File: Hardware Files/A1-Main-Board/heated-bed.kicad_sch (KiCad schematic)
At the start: 16 parts, among them J11 FPC2, J8 FPC_CON, J9 FPC1, Q1 NMOS

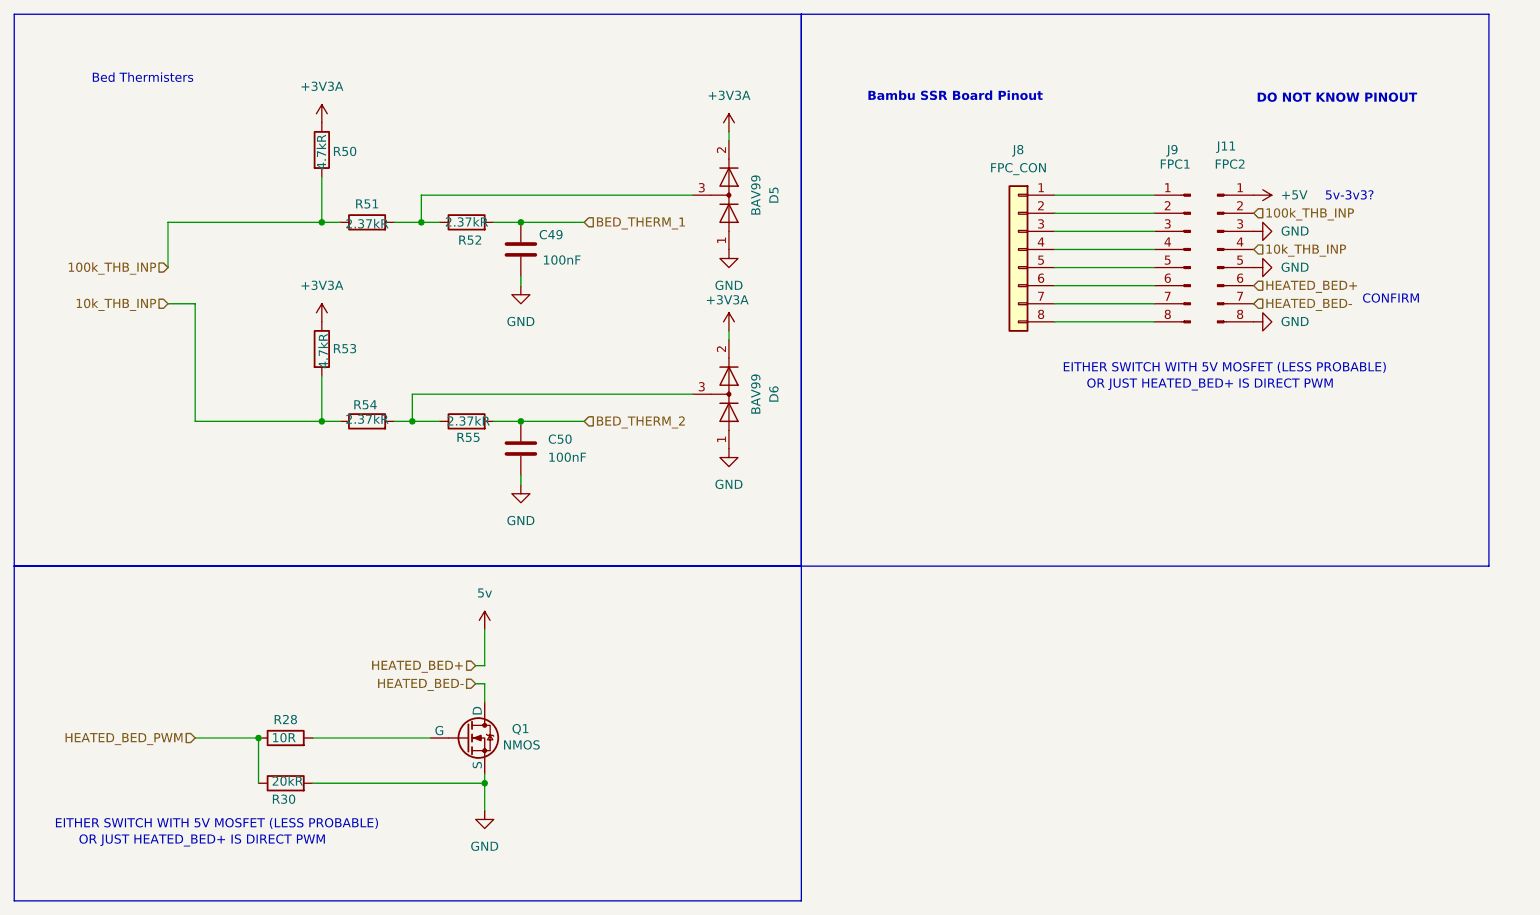
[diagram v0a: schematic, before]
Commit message: e
e
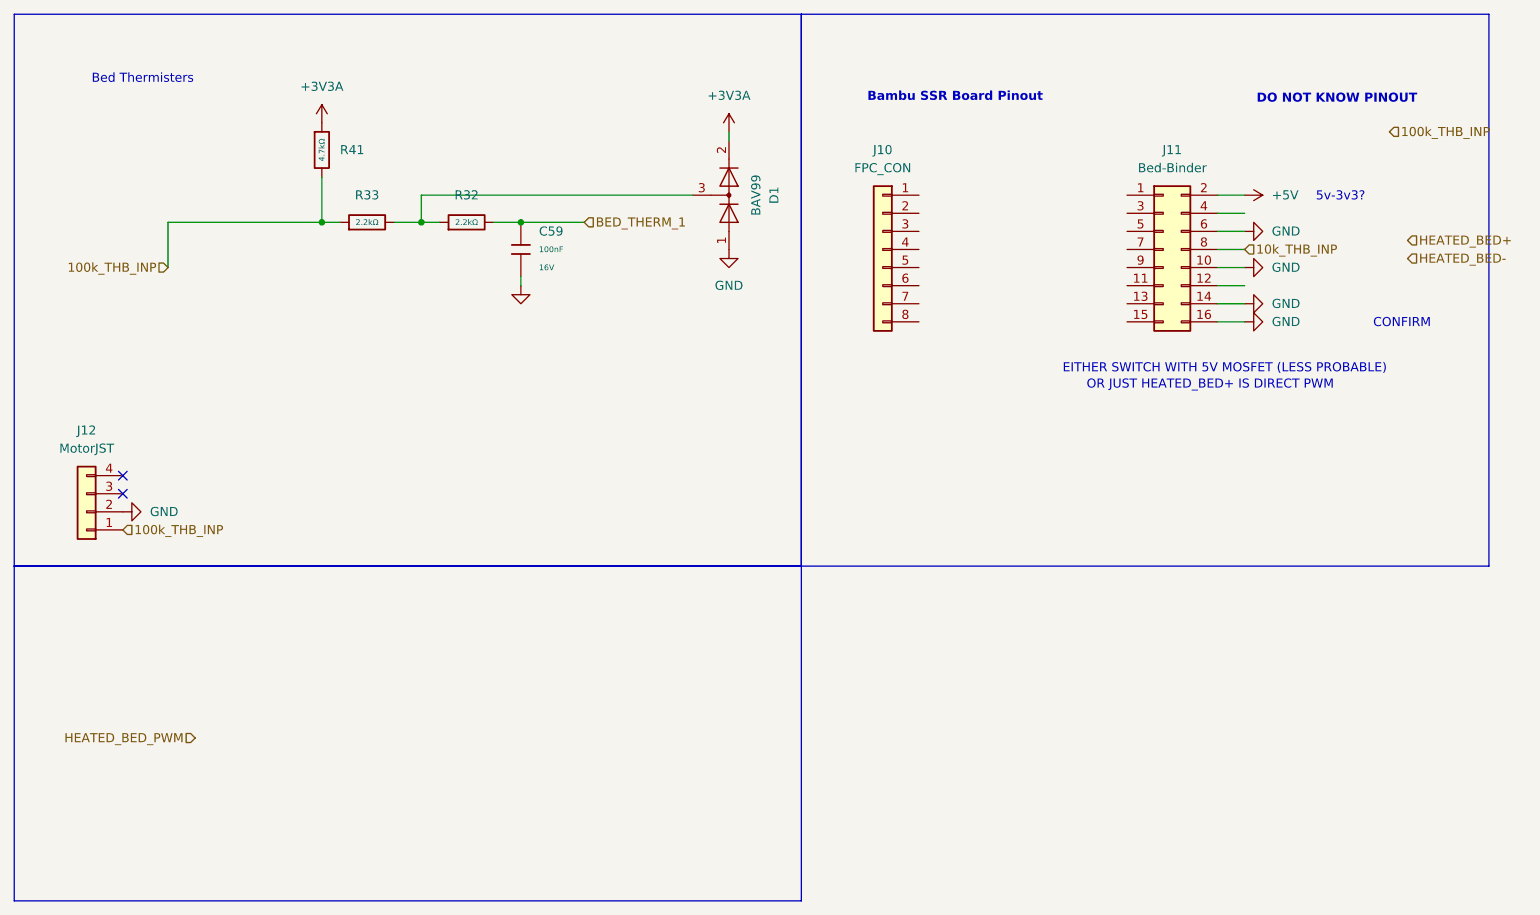
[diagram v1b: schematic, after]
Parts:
- removed C49, C50: 100nF, Capacitor_SMD:C_0402_1005Metric, symbol Device:C
- removed D6: BAV99, Package_TO_SOT_SMD:SOT-23, symbol Diode:BAV99
- removed J11: FPC2, Connector_PinHeader_2.54mm:PinHeader_1x08_P2.54mm_Vertical, symbol Connector:Conn_01x08_Pin
- removed J9: FPC1, Connector_PinHeader_2.54mm:PinHeader_1x08_P2.54mm_Vertical, symbol Connector:Conn_01x08_Pin
- removed Q1: NMOS, Package_TO_SOT_SMD:SOT-23-3, symbol Simulation_SPICE:NMOS
- removed R28: 10R, Resistor_SMD:R_0402_1005Metric, symbol Device:R
- removed R30: 20kR, Resistor_SMD:R_0402_1005Metric, symbol Device:R
- removed R50, R53: 4.7kR, Resistor_SMD:R_0402_1005Metric, symbol Device:R
- removed R51, R52, R54, R55: 2.37kR, Resistor_SMD:R_0402_1005Metric, symbol Device:R
- added C59: 100nF, PCM_JLCPCB:C_0402, symbol PCM_JLCPCB-Capacitors:0402,100nF
- added J11: Bed-Binder, Connector_PinHeader_2.54mm:PinHeader_2x08_P2.54mm_Vertical, symbol Connector_Generic:Conn_02x08_Odd_Even
- added J12: MotorJST, Connector_JST:JST_XH_B4B-XH-A_1x04_P2.50mm_Vertical, symbol Connector_Generic:Conn_01x04
- added R32, R33: 2.2kΩ, PCM_JLCPCB:R_0402, symbol PCM_JLCPCB-Resistors:0402,2.2kΩ
- added R41: 4.7kΩ, PCM_JLCPCB:R_0402, symbol PCM_JLCPCB-Resistors:0402,4.7kΩ
- J10: renamed from J8; footprint (none) -> Connector_FFC-FPC:Hirose_FH12-8S-0.5SH_1x08-1MP_P0.50mm_Horizontal
- renumbered D5 to D1
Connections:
- net +3V3A: now also R41.1
- net +5V: now also J11.2 (Pin_2)
- net 100k_THB_INP: now also J12.1 (Pin_1), R33.1, R41.2
- net 10k_THB_INP: now also J11.8 (Pin_8)
- net BED_THERM_1: now also C59.1, R32.2
- net GND: now also C59.2, J11.10 (Pin_10), J11.14 (Pin_14), J11.16 (Pin_16), J11.6 (Pin_6), J12.2 (Pin_2)
- net at D1.3 (K): now also R32.1, R33.2
- no-connect marks 0 -> 2
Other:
- moved on the sheet: J10
